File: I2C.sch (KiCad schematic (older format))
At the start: 13 parts, among them J701 Conn_01x04, U701 RCLAMP0524P-N

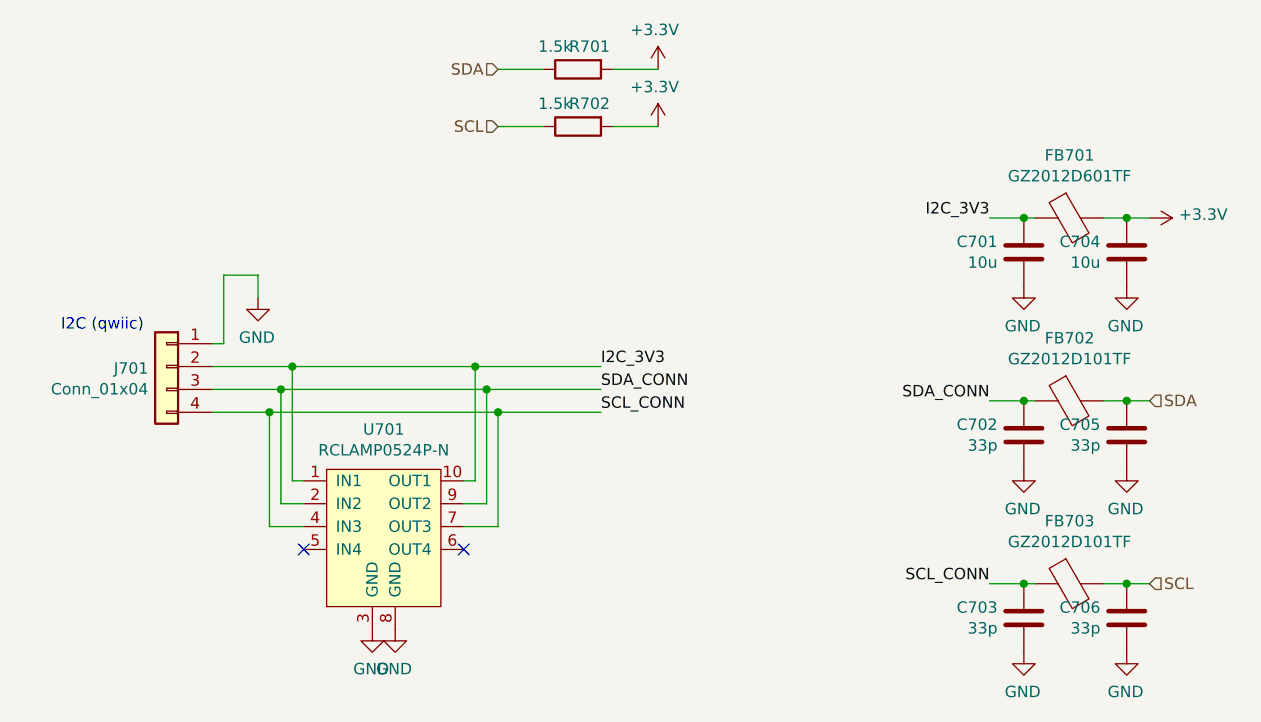
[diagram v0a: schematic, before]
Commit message: Rough PCB layout
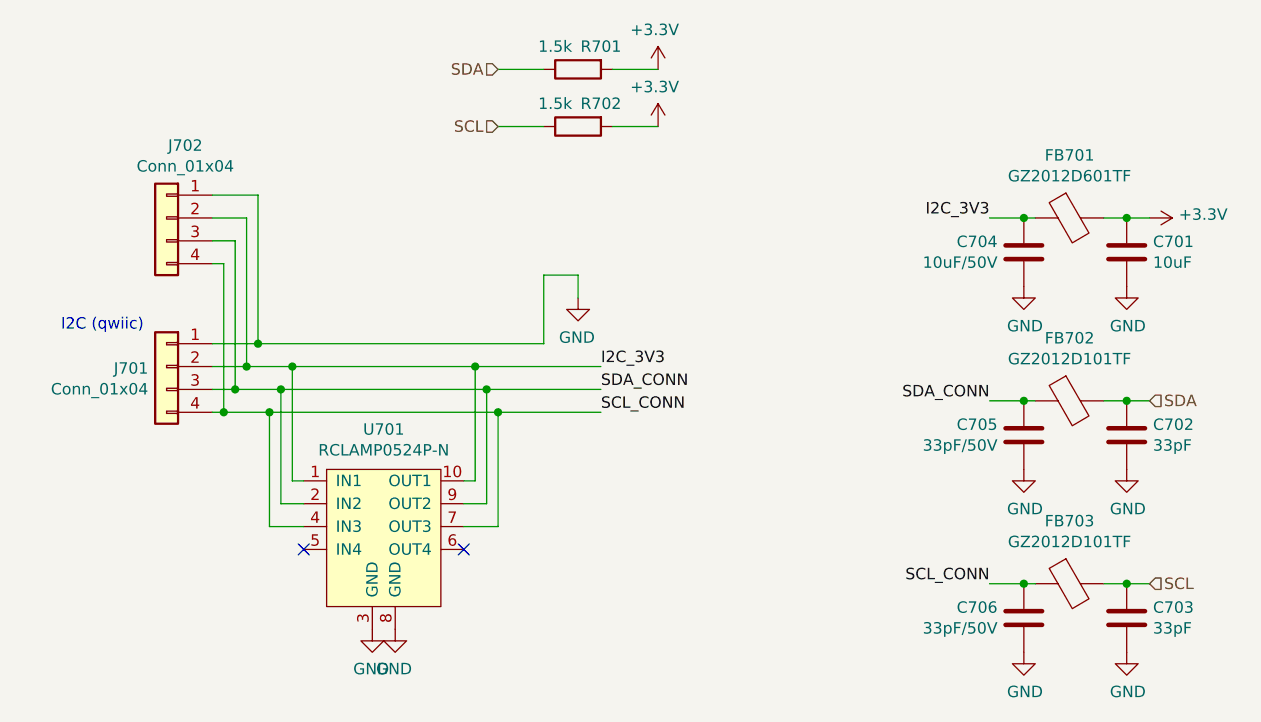
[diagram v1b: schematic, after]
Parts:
- added J702: Conn_01x04, Connector_PinHeader_2.54mm:PinHeader_1x04_P2.54mm_Vertical, symbol Connector_Generic:Conn_01x04
- C701: value 10u -> 10uF; footprint (none) -> Capacitor_SMD:C_0402_1005Metric
- C702, C703: value 33p -> 33pF; footprint (none) -> Capacitor_SMD:C_0402_1005Metric
- C704: value 10u -> 10uF/50V; footprint (none) -> Capacitor_SMD:C_1206_3216Metric
- C705, C706: value 33p -> 33pF/50V; footprint (none) -> Capacitor_SMD:C_0603_1608Metric
- FB701, FB702, FB703: footprint (none) -> Inductor_SMD:L_0805_2012Metric
- J701: footprint (none) -> Connector_JST:JST_SH_BM04B-SRSS-TB_1x04-1MP_P1.00mm_Vertical
- R701, R702: footprint (none) -> Resistor_SMD:R_0402_1005Metric
- U701: footprint (none) -> Package_DFN_QFN:Diodes_UDFN-10_1.0x2.5mm_P0.5mm
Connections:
- net +3V3: now also C701.1; no longer C704.1
- net GND: now also J702.1 (Pin_1)
- net I2C_3V3: now also C704.1, J702.2 (Pin_2); no longer C701.1
- net SCL: now also C703.1; no longer C706.1
- net SCL_CONN: now also C706.1, J702.4 (Pin_4); no longer C703.1
- net SDA: now also C702.1; no longer C705.1
- net SDA_CONN: now also C705.1, J702.3 (Pin_3); no longer C702.1
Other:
- moved on the sheet: C701, C702, C703, C704, C705, C706
